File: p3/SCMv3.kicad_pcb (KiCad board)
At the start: 2 copper layers, 58.7 x 110.9 mm, 127 parts, among them IC1 40106, IC2 40106, IC3 TL082, J1 Conn_01x06, J1-OUT8 JACK-MONO-SWB, J2 Conn_01x02, J2-OUT7 JACK-MONO-SWB, J3 POWER, J3-OUT6 JACK-MONO-SWB, J4 Conn_01x02, J4-OUT5 JACK-MONO-SWB, J5-OUT4 JACK-MONO-SWB, J6-OUT3 JACK-MONO-SWB, J7-OUT2 JACK-MONO-SWB, J8-OUT1 JACK-MONO-SWB, J9-CLK_IN1 JCLK_IN, Q1 Si2318, Q2 Si2318, Q3 Si2318, Q4 Si2318, U1 STM32F030K6Tx, U2 AP7384-33, Y1 16MHz_18pF_FA238

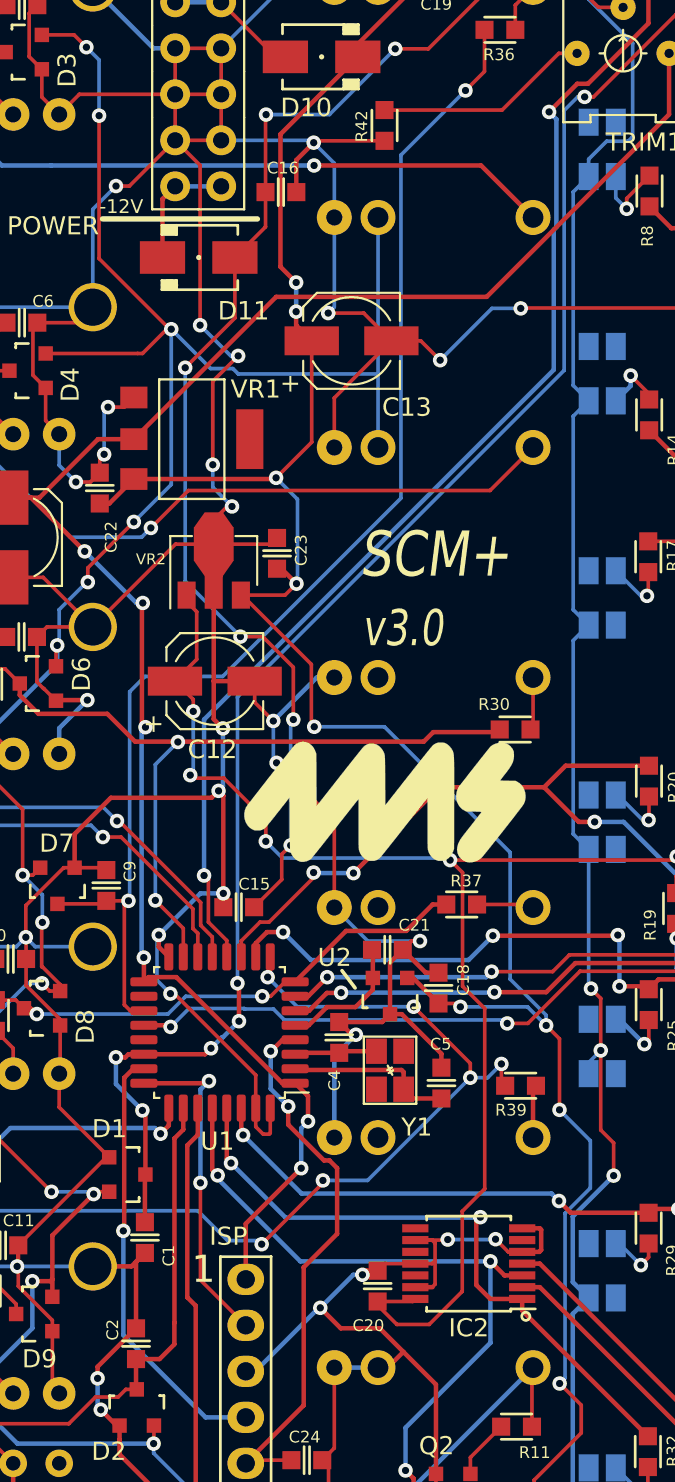
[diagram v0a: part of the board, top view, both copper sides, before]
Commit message: Revert "Merge remote-tracking branch 'origin/main' into main"
This reverts commit 63f0bb0c0b25969e804c40226811b6ef72d39a13.
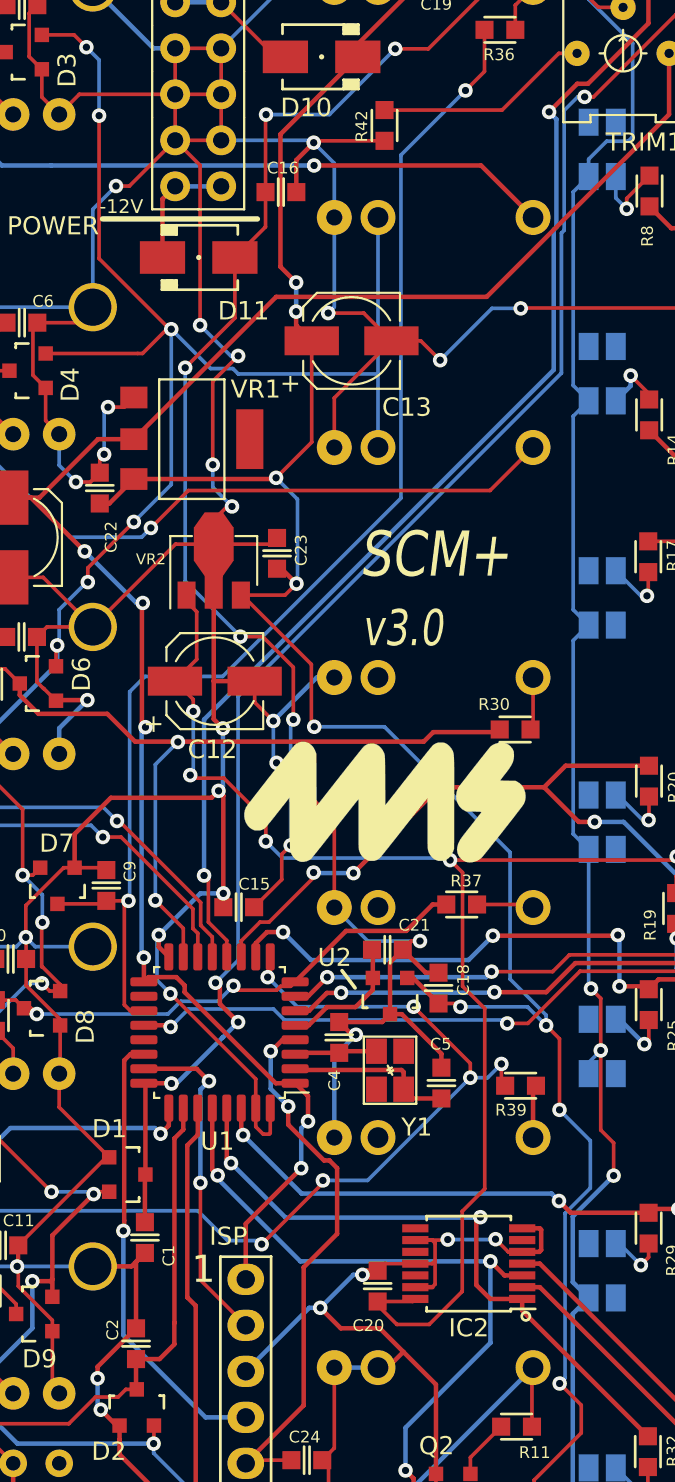
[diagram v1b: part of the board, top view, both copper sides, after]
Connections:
- U1 pad 22: /UC_CLK_IN -> /SWDIO
- U1 pad 23: /SWDIO -> /SWCLK
- U1 pad 24: /SWCLK -> /UC_CLK_IN
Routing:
- net /UC_CLK_IN: track 87.6 -> 85.6 mm, vias 6 -> 4
- net /SWDIO: track 24.2 -> 25.1 mm
